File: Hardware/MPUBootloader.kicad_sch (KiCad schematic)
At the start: 11 parts, among them J6 USB_C_Receptacle_USB2.0_16P, U14 AP2112K-3.3, U17 MKL02Z32VFG4, U18 W25Q64JVSSIM

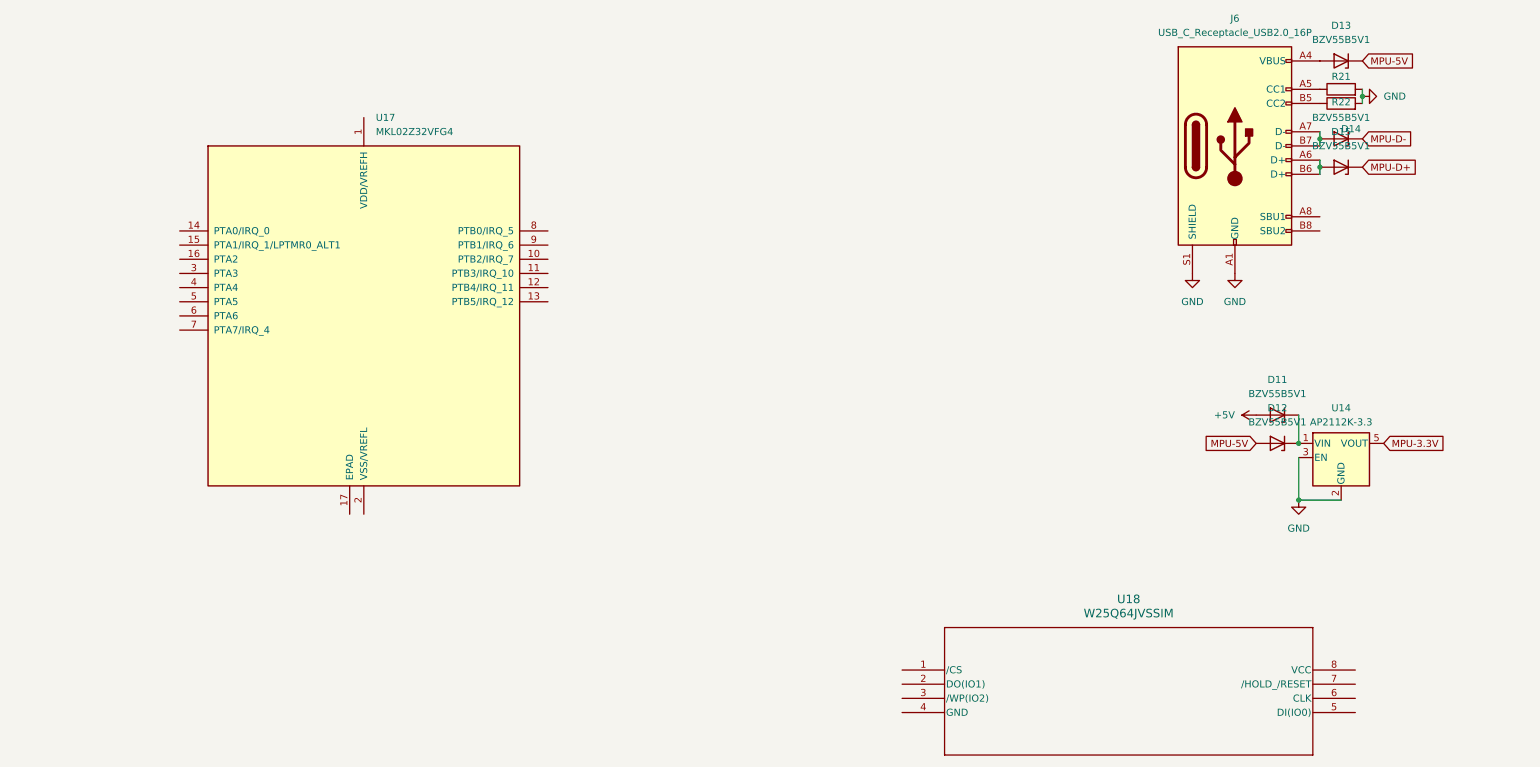
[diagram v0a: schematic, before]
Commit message: 27 feb update
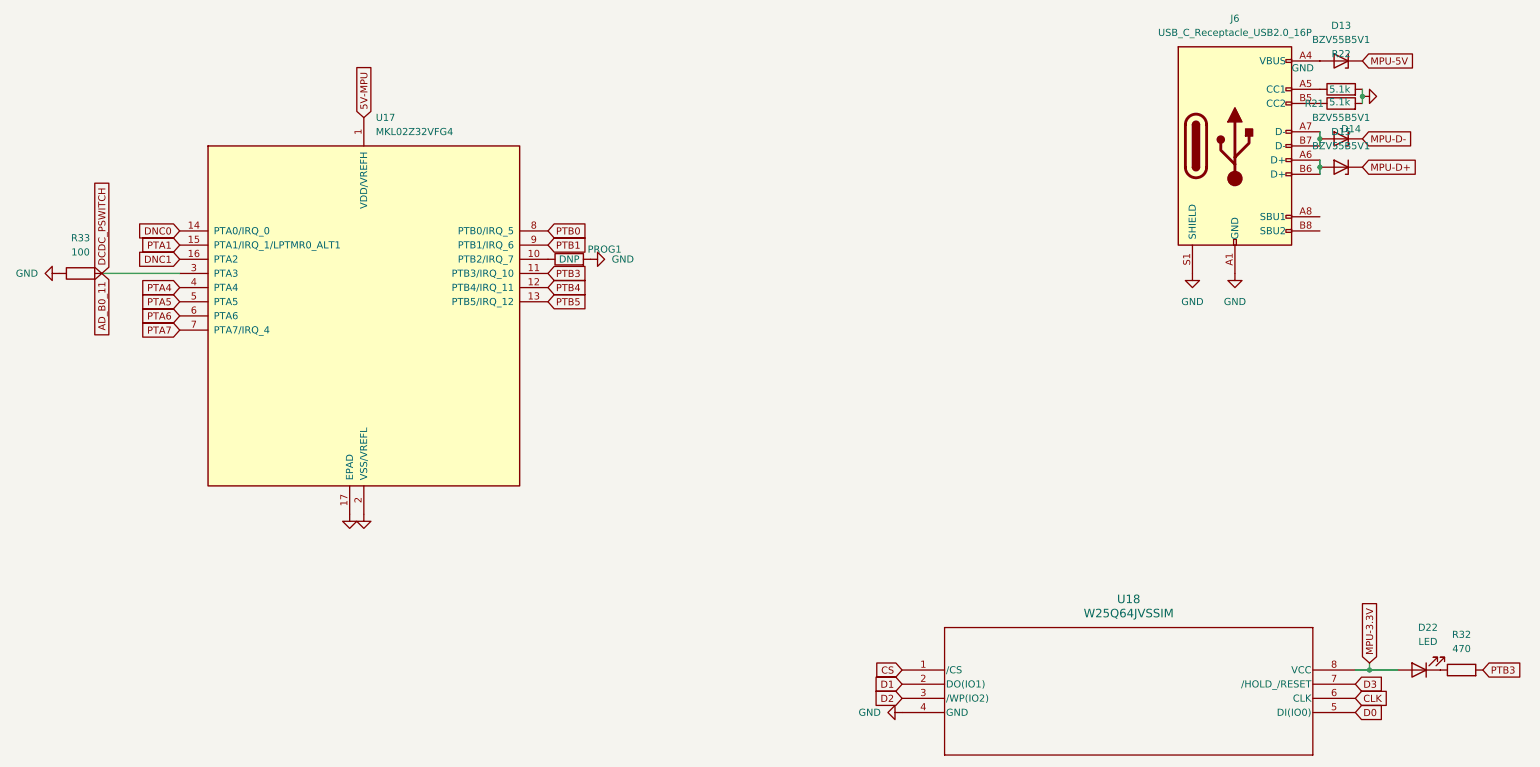
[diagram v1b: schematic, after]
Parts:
- removed D11, D12: BZV55B5V1, Diode_SMD:D_MiniMELF, symbol Diode:BZV55B5V1
- removed U14: AP2112K-3.3, Package_TO_SOT_SMD:SOT-23-5, symbol Regulator_Linear:AP2112K-3.3
- added D22: LED, LED_SMD:LED_1206_3216Metric, symbol Device:LED
- added PROG1: DNP, Resistor_SMD:R_0402_1005Metric_Pad0.72x0.64mm_HandSolder, symbol Device:R
- added R32: 470, Resistor_SMD:R_0201_0603Metric, symbol Device:R
- added R33: 100, Resistor_SMD:R_0201_0603Metric, symbol Device:R
- R21, R22: value R -> 5.1k; footprint Resistor_SMD:R_01005_0402Metric_Pad0.57x0.30mm_HandSolder -> Resistor_SMD:R_0201_0603Metric
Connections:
- net GND: now also U17.17 (EPAD), U17.2 (VSS/VREFL), U18.4 (GND), PROG1.2, R33.1
- net MPU-3.3V: now also U18.8 (VCC), D22.2 (A)
- net at J6.B5 (CC2): now also R21.1; no longer R22.1
- net at J6.A5 (CC1): now also R22.1; no longer R21.1
- net 5V-MPU: now reaches U17.1 (VDD/VREFH)
- net at U17.10 (PTB2/IRQ_7): now also PROG1.1
- net PTB3: now reaches U17.11 (PTB3/IRQ_10)
- net PTB3: now also R32.2
- net PTB4: now reaches U17.12 (PTB4/IRQ_11)
- net PTB5: now reaches U17.13 (PTB5/IRQ_12)
- net DNC0: now reaches U17.14 (PTA0/IRQ_0)
- net PTA1: now reaches U17.15 (PTA1/IRQ_1/LPTMR0_ALT1)
- net DNC1: now reaches U17.16 (PTA2)
- net AD_B0_11: now reaches U17.3 (PTA3)
- net AD_B0_11: now also R33.2
- net PTA4: now reaches U17.4 (PTA4)
- net PTA5: now reaches U17.5 (PTA5)
- net PTA6: now reaches U17.6 (PTA6)
- net PTA7: now reaches U17.7 (PTA7/IRQ_4)
- net PTB0: now reaches U17.8 (PTB0/IRQ_5)
- net PTB1: now reaches U17.9 (PTB1/IRQ_6)
- net CS: now reaches U18.1 (/CS)
- net D1: now reaches U18.2 (DO(IO1))
- net D2: now reaches U18.3 (/WP(IO2))
- net D0: now reaches U18.5 (DI(IO0))
- net CLK: now reaches U18.6 (CLK)
- net D3: now reaches U18.7 (/HOLD_/RESET)
- new net: D22.1 (K), R32.1

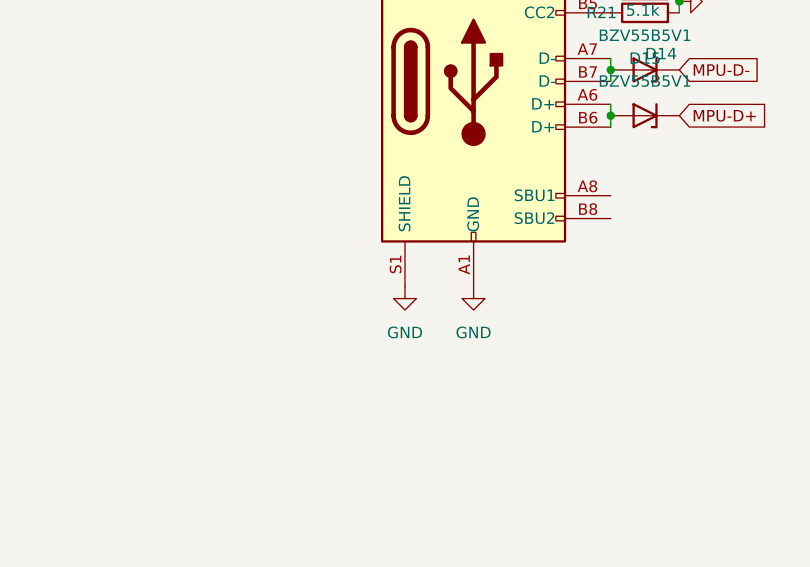
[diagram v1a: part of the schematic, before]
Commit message: 12-March update
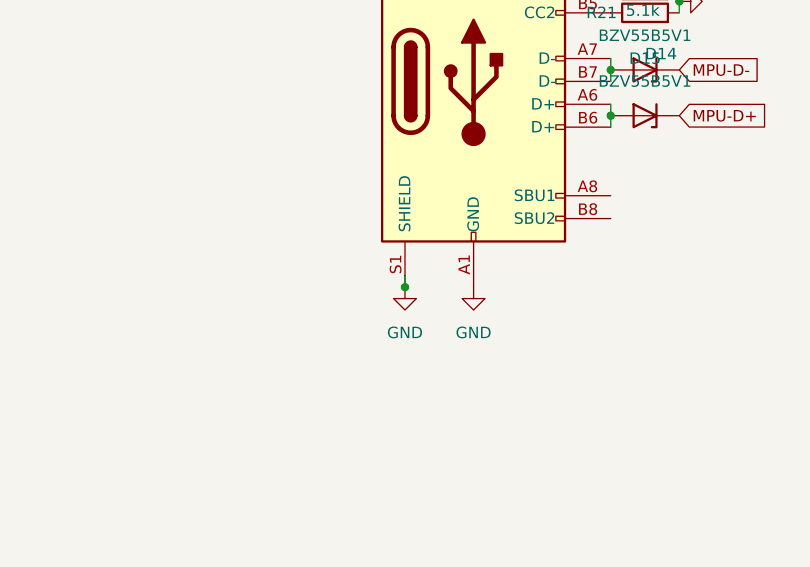
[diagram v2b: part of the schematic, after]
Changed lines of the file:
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@@
+		(color 0 0 0 0)
+	)
+	(junction
+		(at 226.06 72.39)
+		(diameter 0)
 		(color 0 0 0 0)
 	)
@@
 		)
 		(stroke
+			(width 0)
+			(type default)
+		)
+	)
+	(wire
+		(pts
+			(xy 226.06 71.12) (xy 226.06 72.39)
+		)
+		(stroke
